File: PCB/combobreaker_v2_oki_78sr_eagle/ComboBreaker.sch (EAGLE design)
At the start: 9 parts

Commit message: Updated drill size to .35
* Updated drill sizes on most holes to .35
* Adjusted Mini-B USB connector outline on Arduino Nano silkscreen
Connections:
- net GND: now also PWR.-; no longer PWR.GND
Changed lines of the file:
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@@
 <grid distance="0.1" unitdist="inch" unit="inch" style="lines" multiple="1" display="no" altdistance="0.01" altunitdist="inch" altunit="inch"/>
 <layers>
-<layer number="1" name="Top" color="4" fill="1" visible="yes" active="no"/>
-<layer number="2" name="Route2" color="1" fill="3" visible="yes" active="no"/>
-<layer number="3" name="Route3" color="4" fill="3" visible="yes" active="no"/>
-<layer number="4" name="Route4" color="1" fill="4" visible="yes" active="no"/>
-<layer number="5" name="Route5" color="4" fill="4" visible="yes" active="no"/>
-<layer number="6" name="Route6" color="1" fill="8" visible="yes" active="no"/>
-<layer number="7" name="Route7" color="4" fill="8" visible="yes" active="no"/>
-<layer number="8" name="Route8" color="1" fill="2" visible="yes" active="no"/>
-<layer number="9" name="Route9" color="4" fill="2" visible="yes" active="no"/>
-<layer number="10" name="Route10" color="1" fill="7" visible="yes" active="no"/>
-<layer number="11" name="Route11" color="4" fill="7" visible="yes" active="no"/>
-<layer number="12" name="Route12" color="1" fill="5" visible="yes" active="no"/>
-<layer number="13" name="Route13" color="4" fill="5" visible="yes" active="no"/>
-<layer number="14" name="Route14" color="1" fill="6" visible="yes" active="no"/>
-<layer number="15" name="Route15" color="4" fill="6" visible="yes" active="no"/>
-<layer number="16" name="Bottom" color="1" fill="1" visible="yes" active="no"/>
-<layer number="17" name="Pads" color="2" fill="1" visible="yes" active="no"/>
-<layer number="18" name="Vias" color="2" fill="1" visible="yes" active="no"/>
-<layer number="19" name="Unrouted" color="6" fill="1" visible="yes" active="no"/>
-<layer number="20" name="Dimension" color="15" fill="1" visible="yes" active="no"/>
-<layer number="21" name="tPlace" color="7" fill="1" visible="yes" active="no"/>
-<layer number="22" name="bPlace" color="7" fill="1" visible="yes" active="no"/>
-<layer number="23" name="tOrigins" color="15" fill="1" visible="yes" active="no"/>
-<layer number="24" name="bOrigins" color="15" fill="1" visible="yes" active="no"/>
-<layer number="25" name="tNames" color="7" fill="1" visible="yes" active="no"/>
-<layer number="26" name="bNames" color="7" fill="1" visible="yes" active="no"/>
-<layer number="27" name="tValues" color="7" fill="1" visible="yes" active="no"/>
-<layer number="28" name="bValues" color="7" fill="1" visible="yes" active="no"/>
+<layer number="1" name="Top" color="4" fill="1" visible="no" active="no"/>
+<layer number="2" name="Route2" color="1" fill="3" visible="no" active="no"/>
+<layer number="3" name="Route3" color="4" fill="3" visible="no" active="no"/>
+<layer number="4" name="Route4" color="1" fill="4" visible="no" active="no"/>
+<layer number="5" name="Route5" color="4" fill="4" visible="no" active="no"/>
+<layer number="6" name="Route6" color="1" fill="8" visible="no" active="no"/>
+<layer number="7" name="Route7" color="4" fill="8" visible="no" active="no"/>
+<layer number="8" name="Route8" color="1" fill="2" visible="no" active="no"/>
+<layer number="9" name="Route9" color="4" fill="2" visible="no" active="no"/>
+<layer number="10" name="Route10" color="1" fill="7" visible="no" active="no"/>
+<layer number="11" name="Route11" color="4" fill="7" visible="no" active="no"/>
+<layer number="12" name="Route12" color="1" fill="5" visible="no" active="no"/>
+<layer number="13" name="Route13" color="4" fill="5" visible="no" active="no"/>
+<layer number="14" name="Route14" color="1" fill="6" visible="no" active="no"/>
+<layer number="15" name="Route15" color="4" fill="6" visible="no" active="no"/>
+<layer number="16" name="Bottom" color="1" fill="1" visible="no" active="no"/>
+<layer number="17" name="Pads" color="2" fill="1" visible="no" active="no"/>
+<layer number="18" name="Vias" color="2" fill="1" visible="no" active="no"/>
+<layer number="19" name="Unrouted" color="6" fill="1" visible="no" active="no"/>
+<layer number="20" name="Dimension" color="15" fill="1" visible="no" active="no"/>
+<layer number="21" name="tPlace" color="7" fill="1" visible="no" active="no"/>
+<layer number="22" name="bPlace" color="7" fill="1" visible="no" active="no"/>
+<layer number="23" name="tOrigins" color="15" fill="1" visible="no" active="no"/>
+<layer number="24" name="bOrigins" color="15" fill="1" visible="no" active="no"/>
+<layer number="25" name="tNames" color="7" fill="1" visible="no" active="no"/>
+<layer number="26" name="bNames" color="7" fill="1" visible="no" active="no"/>
+<layer number="27" name="tValues" color="7" fill="1" visible="no" active="no"/>
+<layer number="28" name="bValues" color="7" fill="1" visible="no" active="no"/>
 <layer number="29" name="tStop" color="7" fill="3" visible="no" active="no"/>
 <layer number="30" name="bStop" color="7" fill="6" visible="no" active="no"/>
@@
 <layer number="35" name="tGlue" color="7" fill="4" visible="no" active="no"/>
 <layer number="36" name="bGlue" color="7" fill="5" visible="no" active="no"/>
-<layer number="37" name="tTest" color="7" fill="1" visible="yes" active="no"/>
-<layer number="38" name="bTest" color="7" fill="1" visible="yes" active="no"/>
+<layer number="37" name="tTest" color="7" fill="1" visible="no" active="no"/>
+<layer number="38" name="bTest" color="7" fill="1" visible="no" active="no"/>
 <layer number="39" name="tKeepout" color="4" fill="11" visible="no" active="no"/>
 <layer number="40" name="bKeepout" color="1" fill="11" visible="no" active="no"/>
@@
 <layer number="44" name="Drills" color="7" fill="1" visible="no" active="no"/>
 <layer number="45" name="Holes" color="7" fill="1" visible="no" active="no"/>
-<layer number="46" name="Milling" color="3" fill="1" visible="yes" active="no"/>
-<layer number="47" name="Measures" color="7" fill="1" visible="yes" active="no"/>
-<layer number="48" name="Document" color="7" fill="1" visible="yes" active="no"/>
-<layer number="49" name="Reference" color="7" fill="1" visible="yes" active="no"/>
-<layer number="50" name="dxf" color="7" fill="1" visible="yes" active="no"/>
-<layer number="51" name="tDocu" color="7" fill="1" visible="yes" active="no"/>
-<layer number="52" name="bDocu" color="7" fill="1" visible="yes" active="no"/>
-<layer number="53" name="tGND_GNDA" color="7" fill="9" visible="yes" active="no"/>
-<layer number="54" name="bGND_GNDA" color="1" fill="9" visible="yes" active="no"/>
-<layer number="56" name="wert" color="7" fill="1" visible="yes" active="no"/>
-<layer number="57" name="tCAD" color="7" fill="1" visible="yes" active="no"/>
-<layer number="59" name="tCarbon" color="7" fill="1" visible="yes" active="no"/>
-<layer number="60" name="bCarbon" color="7" fill="1" visible="yes" active="no"/>
+<layer number="46" name="Milling" color="3" fill="1" visible="no" active="no"/>
+<layer number="47" name="Measures" color="7" fill="1" visible="no" active="no"/>
+<layer number="48" name="Document" color="7" fill="1" visible="no" active="no"/>
+<layer number="49" name="Reference" color="7" fill="1" visible="no" active="no"/>
+<layer number="50" name="dxf" color="7" fill="1" visible="no" active="no"/>
+<layer number="51" name="tDocu" color="7" fill="1" visible="no" active="no"/>
+<layer number="52" name="bDocu" color="7" fill="1" visible="no" active="no"/>
+<layer number="53" name="tGND_GNDA" color="7" fill="9" visible="no" active="no"/>
+<layer number="54" name="bGND_GNDA" color="1" fill="9" visible="no" active="no"/>
+<layer number="56" name="wert" color="7" fill="1" visible="no" active="no"/>
+<layer number="57" name="tCAD" color="7" fill="1" visible="no" active="no"/>
+<layer number="59" name="tCarbon" color="7" fill="1" visible="no" active="no"/>
+<layer number="60" name="bCarbon" color="7" fill="1" visible="no" active="no"/>
 <layer number="90" name="Modules" color="5" fill="1" visible="yes" active="yes"/>
 <layer number="91" name="Nets" color="2" fill="1" visible="yes" active="yes"/>
@@
 <wire x1="20.32" y1="81.28" x2="-2.54" y2="81.28" width="0.1524" layer="91"/>
 <pinref part="OKI-78SR" gate="G$1" pin="GND"/>
-<pinref part="PWR" gate="G$1" pin="GND"/>
+<pinref part="PWR" gate="G$1" pin="-"/>
 <wire x1="-22.86" y1="86.36" x2="-20.32" y2="86.36" width="0.1524" layer="91"/>
 <wire x1="-20.32" y1="86.36" x2="-20.32" y2="81.28" width="0.1524" layer="91"/>

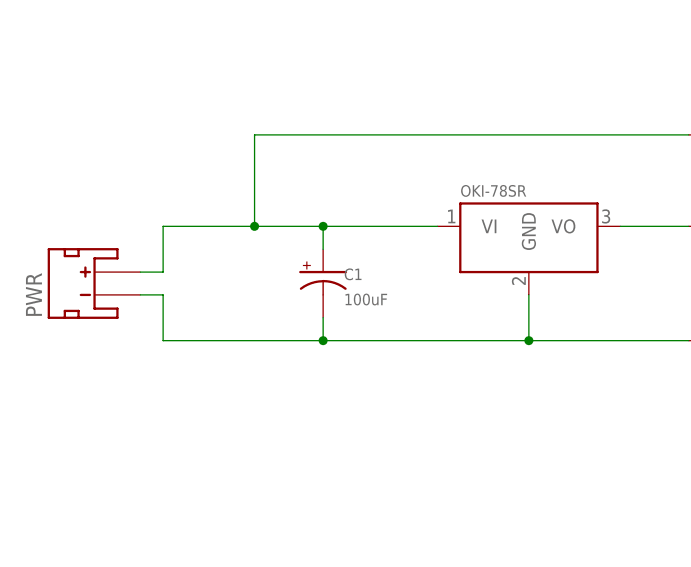
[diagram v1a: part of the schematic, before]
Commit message: v3 PCB
Minor changes
V3 send to fabrication
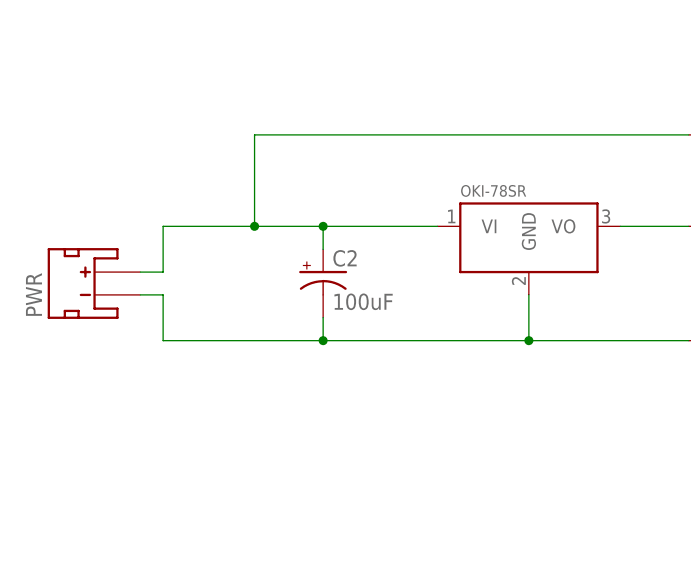
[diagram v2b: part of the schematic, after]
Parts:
- renumbered C1 to C2
